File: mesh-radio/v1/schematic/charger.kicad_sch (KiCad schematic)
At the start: 26 parts, among them J3 S2B-PH-SM4-TB(LF)(SN), Q1 CSD25485F5, Q2 SSM10N954L,EFF, U4 BQ25185DLHR, U5 BQ29700DSER, U6 LM66100DCKR

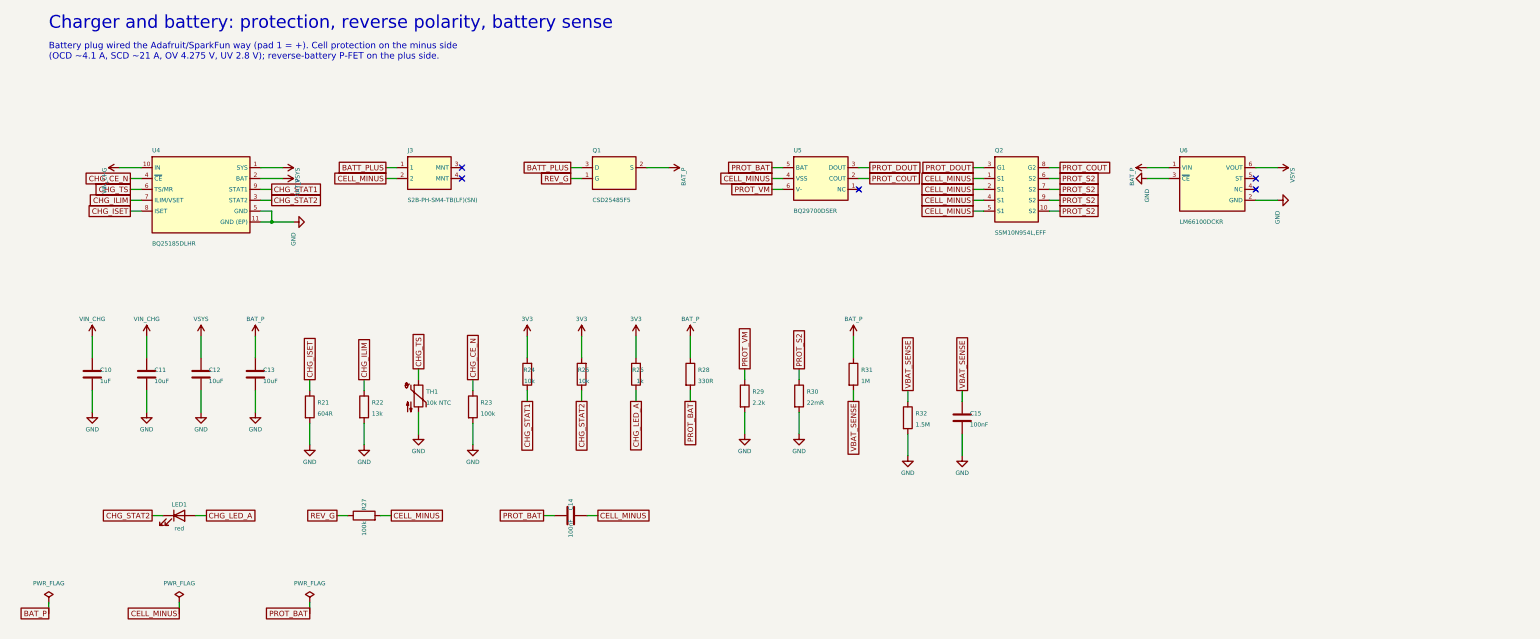
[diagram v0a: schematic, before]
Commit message: Mesh radio v1: power-path and firmware rework in progress (snapshot)
Co-Authored-By: Claude Opus 5.5 <noreply@anthropic.com>
Claude-Session: https://claude.ai/code/session_015TBB2ThqxHSgA8MkFosmn9
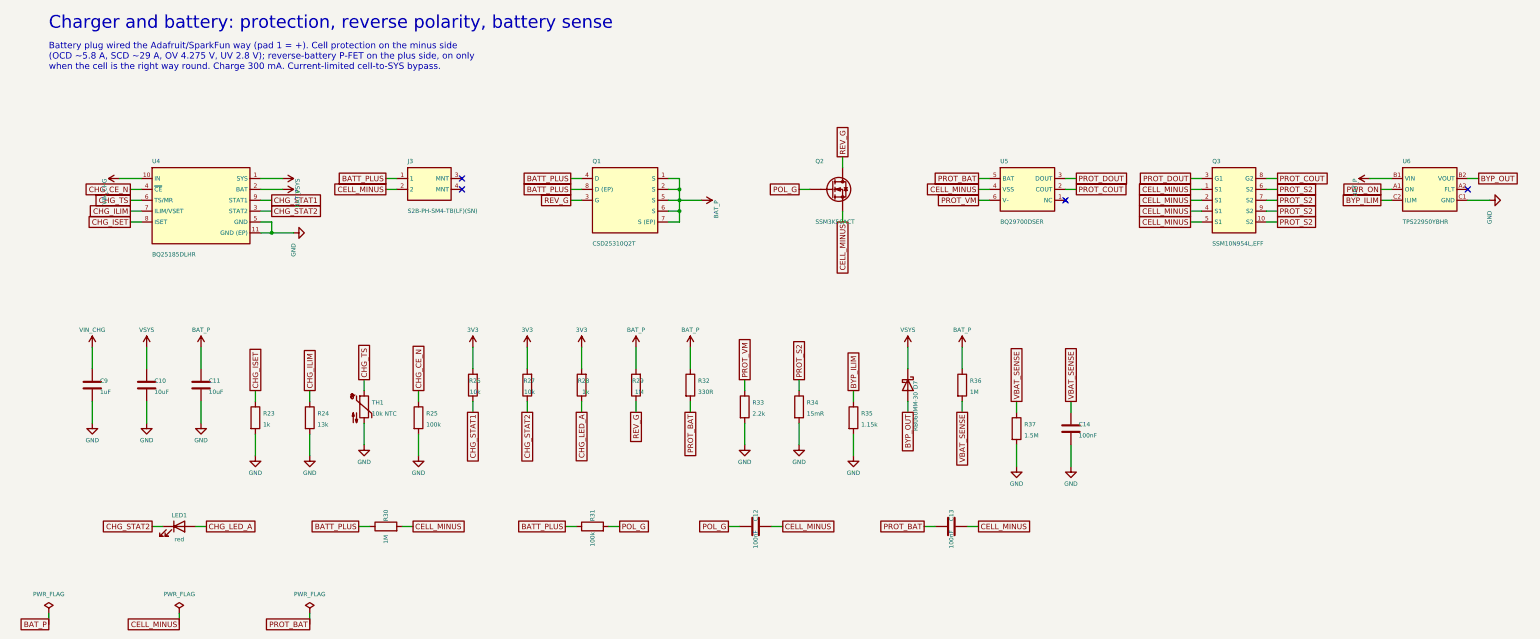
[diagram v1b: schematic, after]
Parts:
- removed C15: 100nF, og:C_0402, symbol Device:C
- removed R21: 604R, og:R_0402, symbol Device:R
- removed R22: 13k, og:R_0402, symbol Device:R
- added C9: 1uF, og:C_0603, symbol Device:C
- added D7: RB060MM-30, og:SOD-123FL, symbol og_device:D_Schottky_RB060MM
- added Q3: SSM10N954L,EFF, og:CSP-10L_SSM10N954L, symbol og:SSM10N954L
- added R33: 2.2k, og:R_0402, symbol Device:R
- added R34: 15mR, og:R_1206, symbol Device:R
- added R35: 1.15k, og:R_0402, symbol Device:R
- added R36: 1M, og:R_0402, symbol Device:R
- added R37: 1.5M, og:R_0402, symbol Device:R
- C10: value 1uF -> 10uF; footprint og:C_0603 -> og:C_0805; DigiKey 1276-1184-1-ND -> 1276-2891-1-ND; LCSC C29936 -> C15850; MPN CL10B105KA8NNNC -> CL21A106KAYNNNE
- C12, C13: value 10uF -> 100nF; footprint og:C_0805 -> og:C_0402; DigiKey 1276-2891-1-ND -> 1276-1001-1-ND; LCSC C15850 -> C1525; MPN CL21A106KAYNNNE -> CL05B104KO5NNNC
- Q1: value CSD25485F5 -> CSD25310Q2T; footprint og:PICOSTAR-3_L1.6-W0.8-P0.53-L -> og:WSON-6_DQK_CSD25310Q2; symbol og:CSD25485F5 -> og:CSD25310Q2; DigiKey 296-47760-1-ND -> 296-50290-1-ND; LCSC C2867111 -> C2871649; MPN CSD25485F5 -> CSD25310Q2T
- Q2: value SSM10N954L,EFF -> SSM3K56ACT; footprint og:CSP-10L_SSM10N954L -> og:SOT-883; symbol og:SSM10N954L -> og_device:Q_NMOS_NMOS; DigiKey 264-SSM10N954LEFFCT-ND -> SSM3K56ACTL3FCT-ND; LCSC C5274420 -> C146308; MPN SSM10N954L,EFF -> SSM3K56ACT,L3F
- R23: value 100k -> 1k; DigiKey 311-100KLRCT-ND -> 311-1.00KLRCT-ND; LCSC C60491 -> C106235; MPN RC0402FR-07100KL -> RC0402FR-071KL
- R24: value 10k -> 13k; DigiKey 311-10.0KLRCT-ND -> 311-13.0KLRCT-ND; LCSC C60490 -> C138057; MPN RC0402FR-0710KL -> RC0402FR-0713KL
- R25: value 10k -> 100k; DigiKey 311-10.0KLRCT-ND -> 311-100KLRCT-ND; LCSC C60490 -> C60491; MPN RC0402FR-0710KL -> RC0402FR-07100KL
- R26: value 1k -> 10k; DigiKey 311-1.00KLRCT-ND -> 311-10.0KLRCT-ND; LCSC C106235 -> C60490; MPN RC0402FR-071KL -> RC0402FR-0710KL
- R27: value 100k -> 10k; DigiKey 311-100KLRCT-ND -> 311-10.0KLRCT-ND; LCSC C60491 -> C60490; MPN RC0402FR-07100KL -> RC0402FR-0710KL
- R28: value 330R -> 1k; DigiKey 311-330LRCT-ND -> 311-1.00KLRCT-ND; LCSC C105875 -> C106235; MPN RC0402FR-07330RL -> RC0402FR-071KL
- R29: value 2.2k -> 1M; DigiKey 311-2.20KLRCT-ND -> 311-1.00MLRCT-ND; LCSC C114762 -> C138033; MPN RC0402FR-072K2L -> RC0402FR-071ML
- R30: value 22mR -> 1M; footprint og:R_1206 -> og:R_0402; DigiKey P.022AUCT-ND -> 311-1.00MLRCT-ND; LCSC C2075813 -> C138033; MPN ERJ-8BWFR022V -> RC0402FR-071ML; Manufacturer Panasonic -> Yageo
- R31: value 1M -> 100k; DigiKey 311-1.00MLRCT-ND -> 311-100KLRCT-ND; LCSC C138033 -> C60491; MPN RC0402FR-071ML -> RC0402FR-07100KL
- R32: value 1.5M -> 330R; DigiKey 13-RC0402FR-071M5LCT-ND -> 311-330LRCT-ND; LCSC C138034 -> C105875; MPN RC0402FR-071M5L -> RC0402FR-07330RL
- U6: value LM66100DCKR -> TPS22950YBHR; footprint og:SC-70-6 -> og:DSBGA-6_L1.2-W0.8-R2-C3-P0.40-BL; symbol og:LM66100 -> og:TPS22950; DigiKey (none) -> 296-TPS22950YBHRCT-ND; LCSC C2869734 -> C3230039; MPN LM66100DCKR -> TPS22950YBHR
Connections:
- net 3V3: now also R27.2, R28.2; no longer R24.2, R25.2
- net BATT_PLUS: now also Q1.4 (D), Q1.8 (D (EP)), R30.1, R31.1; no longer Q1.3 (D)
- net BAT_P: now also C11.1, Q1.1 (S), Q1.5 (S), Q1.6 (S), Q1.7 (S (EP)), R29.2, R32.1, U6.B1 (VIN), R36.1; no longer C13.1, R28.1, R31.1, U6.1 (VIN)
- net CELL_MINUS: now also C12.2, C13.2, R30.2, Q3.1 (S1), Q3.2 (S1), Q3.4 (S1), Q3.5 (S1); no longer C14.2, Q2.1 (S1), Q2.4 (S1), Q2.5 (S1), R27.2
- net CHG_CE_N: now also R25.1; no longer R23.1
- net CHG_ILIM: now also R24.1
- net CHG_ISET: now also R23.1
- net CHG_LED_A: now also R28.1; no longer R26.1
- net CHG_STAT1: now also R26.1; no longer R24.1
- net CHG_STAT2: now also R27.1; no longer R25.1
- net GND: now also C14.2, R24.2, R25.2, U6.C1 (GND), C9.2, R33.2, R34.2, R35.2, R37.2; no longer C12.2, C13.2, R29.2, R30.2, R32.2, U6.2 (GND), U6.3 (~{CE})
- net PROT_BAT: now also C13.1, R32.2; no longer C14.1, R28.2
- net PROT_COUT: now also Q3.8 (G2); no longer Q2.8 (G2)
- net PROT_DOUT: now also Q3.3 (G1); no longer Q2.3 (G1)
- net PROT_S2: now also Q3.10 (S2), Q3.6 (S2), Q3.7 (S2), Q3.9 (S2), R34.1; no longer Q2.10 (S2), Q2.6 (S2), Q2.7 (S2), Q2.9 (S2), R30.1
- net PROT_VM: now also R33.1; no longer R29.1
- net REV_G: now also Q1.3 (G), Q2.3 (D), R29.1; no longer Q1.1 (G), R27.1
- net VBAT_SENSE: now also C14.1, R36.2, R37.1; no longer R31.2, R32.1
- net VIN_CHG: now also C9.1; no longer C10.1, C11.1
- net VSYS: now also C10.1, D7.1 (K); no longer C12.1, U6.6 (VOUT)
- new net BYP_ILIM: R35.1, U6.C2 (ILIM)
- new net BYP_OUT: D7.2 (A), U6.B2 (VOUT)
- new net POL_G: C12.1, Q2.1 (G), R31.2
- new net PWR_ON: U6.A1 (ON)
- no-connect marks 5 -> 4
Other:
- note added: "Battery plug wired the Adafruit/SparkFun way (pad 1 = +). Cell protection on the minus side (OCD ~5.8 A, SCD ~29 A, OV 4.275 V, UV 2.8 V); reverse-battery P-FET on the plus side, on only when the cell is the right way round. Charge 300 mA. Current-limited cell-to-SYS bypass."
- note removed: "Battery plug wired the Adafruit/SparkFun way (pad 1 = +). Cell protection on the minus side (OCD ~4.1 A, SCD ~21 A, OV 4.275 V, UV 2.8 V); reverse-battery P-FET on the plus side."
- moved on the sheet: C10, C11, C12, C13, C14, J3, LED1, R23, R24, R25, R26, R27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
